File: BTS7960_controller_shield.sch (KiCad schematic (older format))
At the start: 39 parts, among them J1 Conn_ST_STDC14, J2 Conn_02x04_Odd_Even, J3 USB_C_Receptacle_USB2.0, J4 Conn_01x04, J5 USB_C_Receptacle_USB2.0, J6 Conn_ST_STDC14, J7 Conn_01x02, Q1 BTN8982TA, Q2 BTN8982TA, U1 LDFM33PVR, U2 STM32F302K8Ux, U3 USBLC6-2SC6, Y1 16MHz

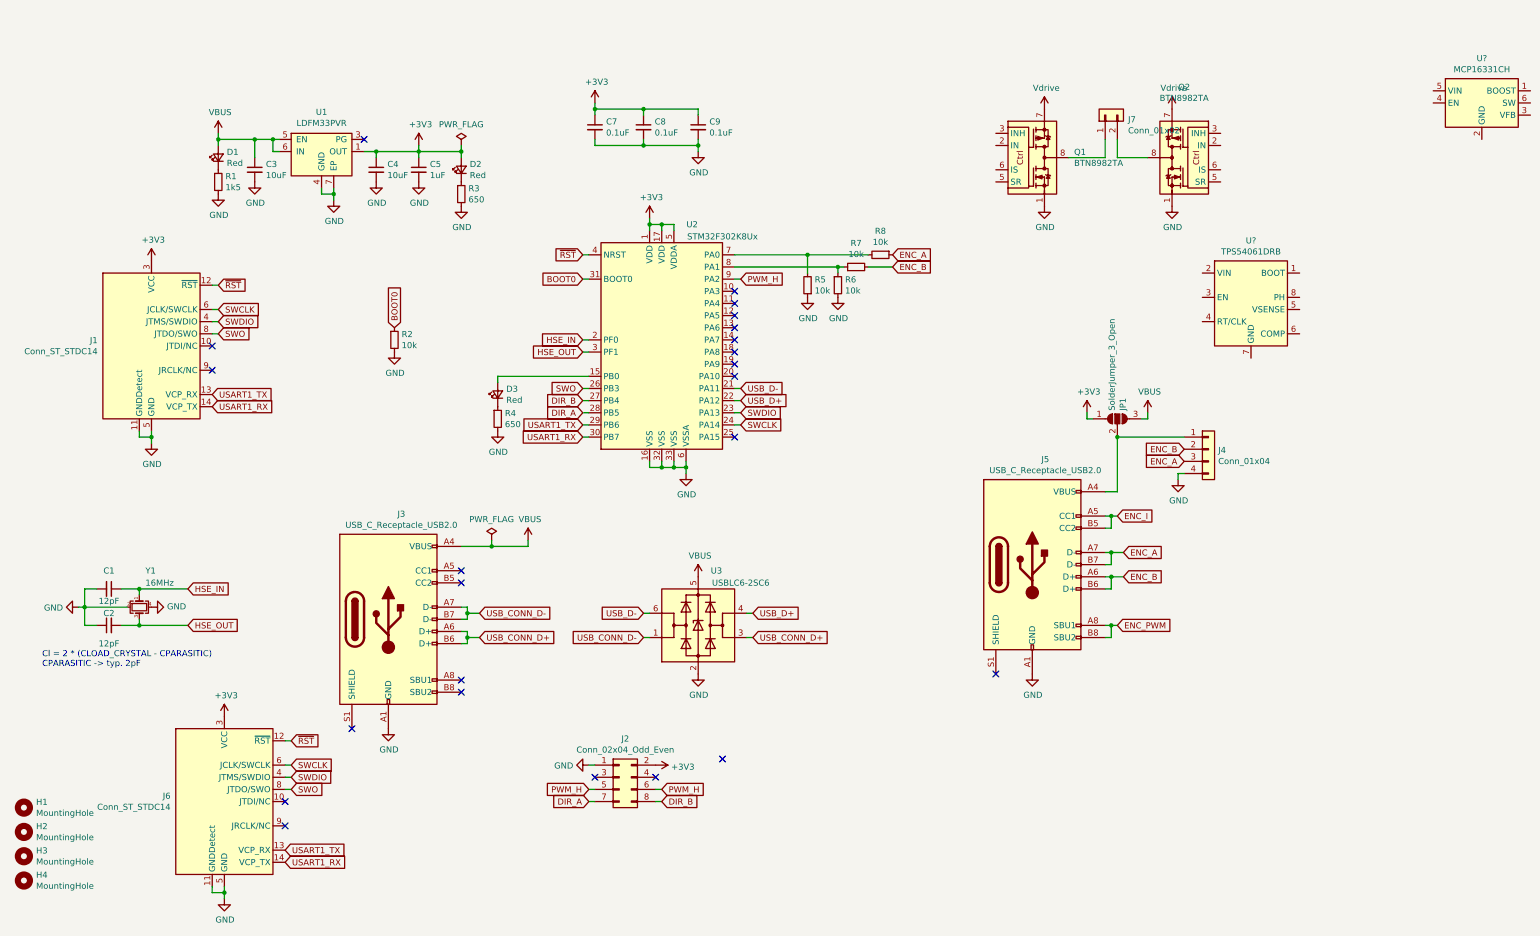
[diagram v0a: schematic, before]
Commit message: New idea
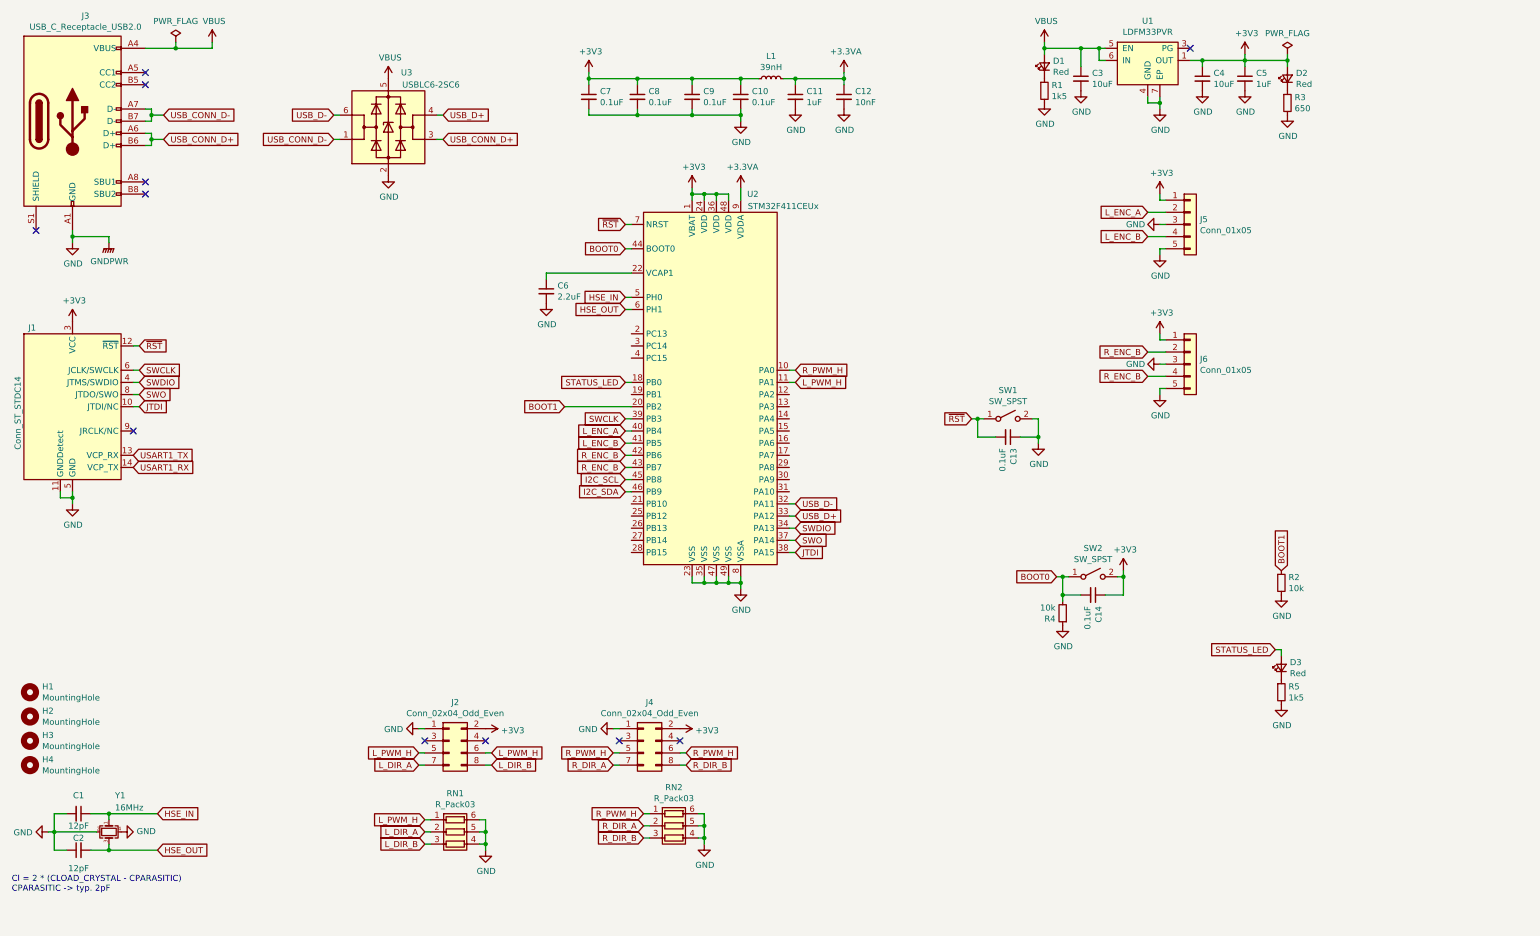
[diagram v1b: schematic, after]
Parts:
- removed J4: Conn_01x04, TerminalBlock_TE-Connectivity:TerminalBlock_TE_282834-4_1x04_P2.54mm_Horizontal, symbol Connector_Generic:Conn_01x04
- removed J5: USB_C_Receptacle_USB2.0, Connector_USB:USB_C_Receptacle_XKB_U262-16XN-4BVC11, symbol Connector:USB_C_Receptacle_USB2.0
- removed J6: Conn_ST_STDC14, Connector:Tag-Connect_TC2070-IDC-FP_2x07_P1.27mm_Vertical, symbol Connector:Conn_ST_STDC14
- removed J7: Conn_01x02, symbol Connector_Generic:Conn_01x02
- removed JP1: SolderJumper_3_Open, Jumper:SolderJumper-3_P2.0mm_Open_TrianglePad1.0x1.5mm_NumberLabels, symbol Jumper:SolderJumper_3_Open
- removed Q1, Q2: BTN8982TA, Package_TO_SOT_SMD:TO-263-7_TabPin8, symbol Power_Management:BTN8982TA
- removed R6, R7, R8: 10k, Resistor_SMD:R_0402_1005Metric_Pad0.72x0.64mm_HandSolder, symbol Device:R_Small
- removed U2: STM32F302K8Ux, Package_DFN_QFN:QFN-32-1EP_5x5mm_P0.5mm_EP3.45x3.45mm, symbol MCU_ST_STM32F3:STM32F302K8Ux
- removed U?: TPS54061DRB, Package_SON:Texas_S-PVSON-N8, symbol Regulator_Switching:TPS54061DRB
- removed U?: MCP16331CH, Package_TO_SOT_SMD:SOT-23-6, symbol Regulator_Switching:MCP16331CH
- added C10, C13, C14: 0.1uF, Capacitor_SMD:C_0402_1005Metric_Pad0.74x0.62mm_HandSolder, symbol Device:C_Small
- added C11: 1uF, Capacitor_SMD:C_0402_1005Metric_Pad0.74x0.62mm_HandSolder, symbol Device:C_Small
- added C12: 10nF, Capacitor_SMD:C_0402_1005Metric_Pad0.74x0.62mm_HandSolder, symbol Device:C_Small
- added C6: 2.2uF, Capacitor_SMD:C_0402_1005Metric_Pad0.74x0.62mm_HandSolder, symbol Device:C_Small
- added J4: Conn_02x04_Odd_Even, Connector_PinSocket_2.54mm:PinSocket_2x04_P2.54mm_Vertical, symbol Connector_Generic:Conn_02x04_Odd_Even
- added J5, J6: Conn_01x05, Connector_JST:JST_PH_S5B-PH-K_1x05_P2.00mm_Horizontal, symbol Connector_Generic:Conn_01x05
- added L1: 39nH, Inductor_SMD:L_0603_1608Metric, symbol Device:L_Small
- added RN1, RN2: R_Pack03, Package_DIP:DIP-6_W8.89mm_SMDSocket_LongPads, symbol Device:R_Pack03
- added SW1, SW2: SW_SPST, Button_Switch_THT:SW_Tactile_SPST_Angled_PTS645Vx58-2LFS, symbol Switch:SW_SPST
- added U2: STM32F411CEUx, Package_DFN_QFN:QFN-48-1EP_7x7mm_P0.5mm_EP5.6x5.6mm, symbol MCU_ST_STM32F4:STM32F411CEUx
- R4: value 650 -> 10k
- R5: value 10k -> 1k5
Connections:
- net +3V3: now also C10.1, C14.1, J4.2 (Pin_2), J5.1 (Pin_1), J6.1 (Pin_1), L1.1, SW2.2 (B), U2.1 (VBAT), U2.24 (VDD), U2.36 (VDD), U2.48 (VDD)
- net BOOT0: now also R4.2, C14.2, SW2.1 (A), U2.44 (BOOT0); no longer R2.1
- net GND: now also R4.1, R5.2, C10.2, C11.2, C12.2, C13.1, C6.2, J4.1 (Pin_1), J5.3 (Pin_3), J5.5 (Pin_5), J6.3 (Pin_3), J6.5 (Pin_5), RN1.4 (R3.2), RN1.5 (R2.2), RN1.6 (R1.2), RN2.4 (R3.2), RN2.5 (R2.2), RN2.6 (R1.2), SW1.2 (B), U2.23 (VSS), U2.35 (VSS), U2.47 (VSS), U2.49 (VSS), U2.8 (VSSA); no longer R4.2, R5.1
- net HSE_IN: now also U2.5 (PH0)
- net HSE_OUT: now also U2.6 (PH1)
- net SWCLK: now also U2.39 (PB3)
- net SWDIO: now also U2.34 (PA13)
- net SWO: now also U2.37 (PA14)
- net USB_D+: now also U2.33 (PA12)
- net USB_D-: now also U2.32 (PA11)
- net ~RST: now also C13.2, SW1.1 (A), U2.7 (NRST)
- net STATUS_LED: now reaches D3.2 (A)
- net STATUS_LED: now also U2.18 (PB0)
- net JTDI: now reaches J1.10 (JTDI/NC)
- net JTDI: now also U2.38 (PA15)
- net at D3.1 (K): now also R5.1; no longer R4.1
- net DIR_A renamed L_DIR_A
- net L_DIR_A: now also RN1.2 (R2.1)
- net DIR_B renamed L_DIR_B
- net L_DIR_B: now also RN1.3 (R3.1)
- net PWM_H renamed L_PWM_H
- net L_PWM_H: now also RN1.1 (R1.1), U2.11 (PA1)
- new net: C6.1, U2.22 (VCAP1)
- new net +3.3VA: C11.1, C12.1, L1.2, U2.9 (VDDA)
- new net BOOT1: R2.1, U2.20 (PB2)
- new net I2C_SCL: U2.45 (PB8)
- new net I2C_SDA: U2.46 (PB9)
- new net L_ENC_A: J5.2 (Pin_2), U2.40 (PB4)
- new net L_ENC_B: J5.4 (Pin_4), U2.41 (PB5)
- new net R_DIR_A: J4.7 (Pin_7), RN2.2 (R2.1)
- new net R_DIR_B: J4.8 (Pin_8), RN2.3 (R3.1)
- new net R_ENC_B: J6.2 (Pin_2), J6.4 (Pin_4), U2.42 (PB6), U2.43 (PB7)
- new net R_PWM_H: J4.5 (Pin_5), J4.6 (Pin_6), RN2.1 (R1.1), U2.10 (PA0)
- no-connect marks 23 -> 11
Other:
- moved on the sheet: C1, C2, C3, C4, C5, C7, C8, C9, D1, D2, H1, H2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

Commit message: Przygotowanie do projektu
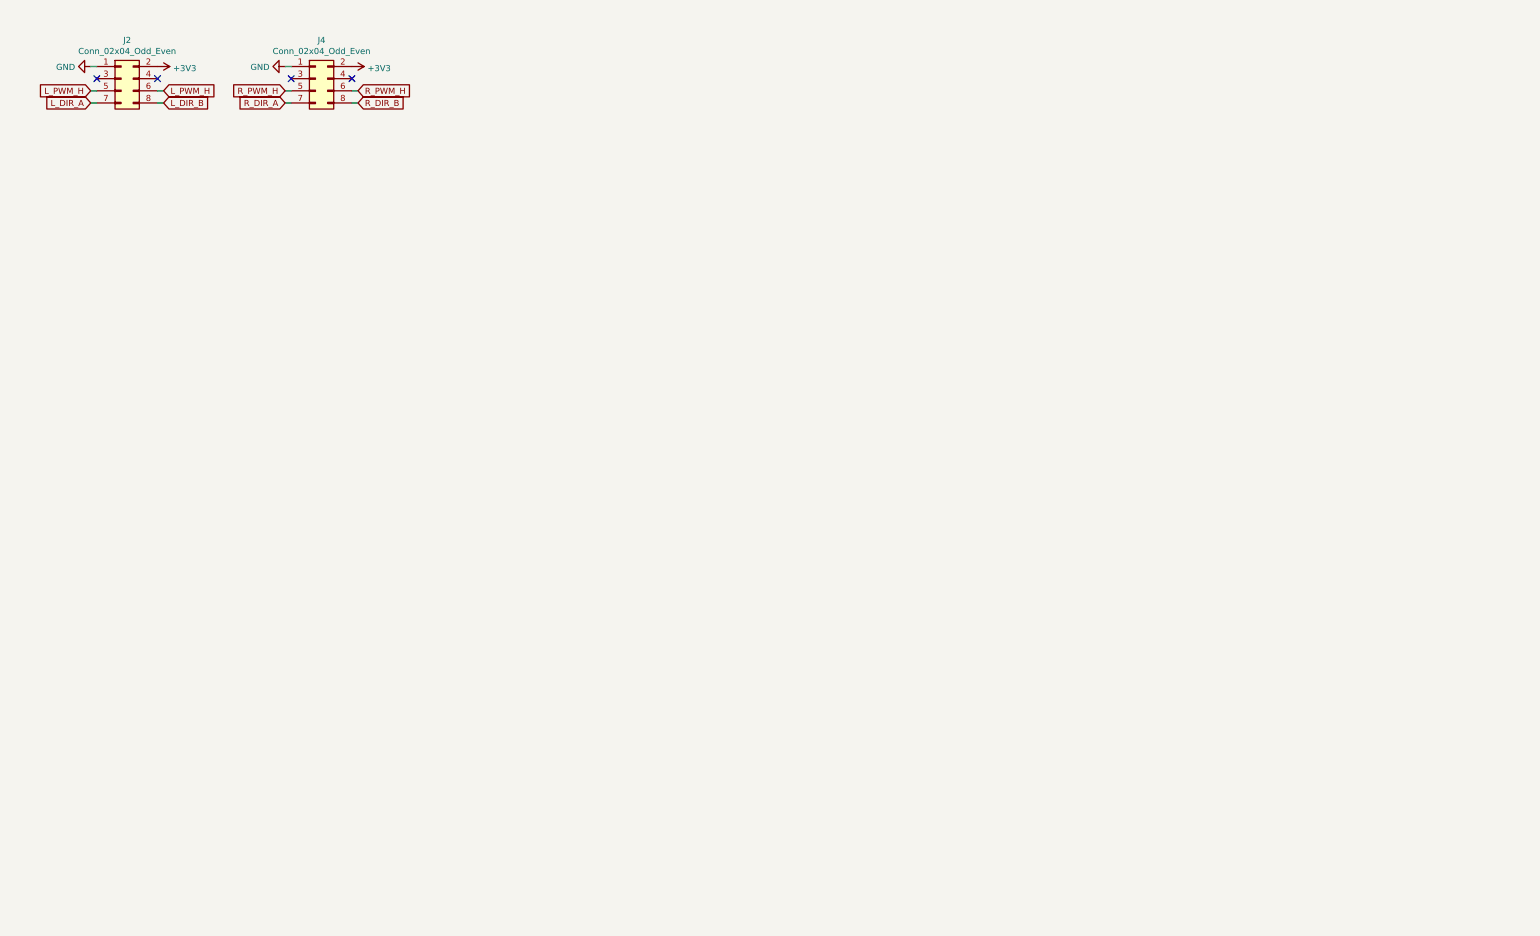
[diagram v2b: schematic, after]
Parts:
- removed C1, C2: 12pF, Capacitor_SMD:C_0402_1005Metric_Pad0.74x0.62mm_HandSolder, symbol Device:C_Small
- removed C10, C13, C14, C7, C8, C9: 0.1uF, Capacitor_SMD:C_0402_1005Metric_Pad0.74x0.62mm_HandSolder, symbol Device:C_Small
- removed C11: 1uF, Capacitor_SMD:C_0402_1005Metric_Pad0.74x0.62mm_HandSolder, symbol Device:C_Small
- removed C12: 10nF, Capacitor_SMD:C_0402_1005Metric_Pad0.74x0.62mm_HandSolder, symbol Device:C_Small
- removed C3, C4: 10uF, Capacitor_SMD:C_0603_1608Metric_Pad1.08x0.95mm_HandSolder, symbol Device:C_Small
- removed C5: 1uF, Capacitor_SMD:C_0603_1608Metric_Pad1.08x0.95mm_HandSolder, symbol Device:C_Small
- removed C6: 2.2uF, Capacitor_SMD:C_0402_1005Metric_Pad0.74x0.62mm_HandSolder, symbol Device:C_Small
- removed D1, D2, D3: Red, LED_SMD:LED_0603_1608Metric_Pad1.05x0.95mm_HandSolder, symbol Device:LED_Small
- removed H1, H2, H3, H4: MountingHole, MountingHole:MountingHole_3.2mm_M3, symbol Mechanical:MountingHole
- removed J1: Conn_ST_STDC14, Connector_PinHeader_1.27mm:PinHeader_2x07_P1.27mm_Vertical_SMD, symbol Connector:Conn_ST_STDC14
- removed J3: USB_C_Receptacle_USB2.0, Connector_USB:USB_C_Receptacle_XKB_U262-16XN-4BVC11, symbol Connector:USB_C_Receptacle_USB2.0
- removed J5, J6: Conn_01x05, Connector_JST:JST_PH_S5B-PH-K_1x05_P2.00mm_Horizontal, symbol Connector_Generic:Conn_01x05
- removed L1: 39nH, Inductor_SMD:L_0603_1608Metric, symbol Device:L_Small
- removed R1, R5: 1k5, Resistor_SMD:R_0402_1005Metric_Pad0.72x0.64mm_HandSolder, symbol Device:R_Small
- removed R2, R4: 10k, Resistor_SMD:R_0402_1005Metric_Pad0.72x0.64mm_HandSolder, symbol Device:R_Small
- removed R3: 650, Resistor_SMD:R_0402_1005Metric_Pad0.72x0.64mm_HandSolder, symbol Device:R_Small
- removed RN1, RN2: R_Pack03, Package_DIP:DIP-6_W8.89mm_SMDSocket_LongPads, symbol Device:R_Pack03
- removed SW1, SW2: SW_SPST, Button_Switch_THT:SW_Tactile_SPST_Angled_PTS645Vx58-2LFS, symbol Switch:SW_SPST
- removed U1: LDFM33PVR, Package_DFN_QFN:DFN-6-1EP_2x2mm_P0.5mm_EP0.61x1.42mm, symbol synermycha-electronics:LDFM33PVR
- removed U2: STM32F411CEUx, Package_DFN_QFN:QFN-48-1EP_7x7mm_P0.5mm_EP5.6x5.6mm, symbol MCU_ST_STM32F4:STM32F411CEUx
- removed U3: USBLC6-2SC6, Package_TO_SOT_SMD:SOT-23-6, symbol Power_Protection:USBLC6-2SC6
- removed Y1: 16MHz, Crystal:Crystal_SMD_Abracon_ABM10-4Pin_2.5x2.0mm, symbol Device:Crystal_GND24_Small
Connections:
- no-connect marks 11 -> 4
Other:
- note removed: "Cl = 2 * (CLOAD_CRYSTAL - CPARASITIC)\nCPARASITIC -> typ. 2pF"
- moved on the sheet: J2, J4
